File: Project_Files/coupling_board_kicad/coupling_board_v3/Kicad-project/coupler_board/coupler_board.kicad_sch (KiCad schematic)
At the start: 26 parts, among them IC1 ISO6741DWR, IC2 ISO6740FDWR, IC3 ISO6740FDWR, J1 Molex Microfit, J2 Conn_02x12_Odd_Even, J3 Molex6, J5 DB25_Socket, J7 Molex Microfit, J8 Molex Microfit, J9 Molex Microfit

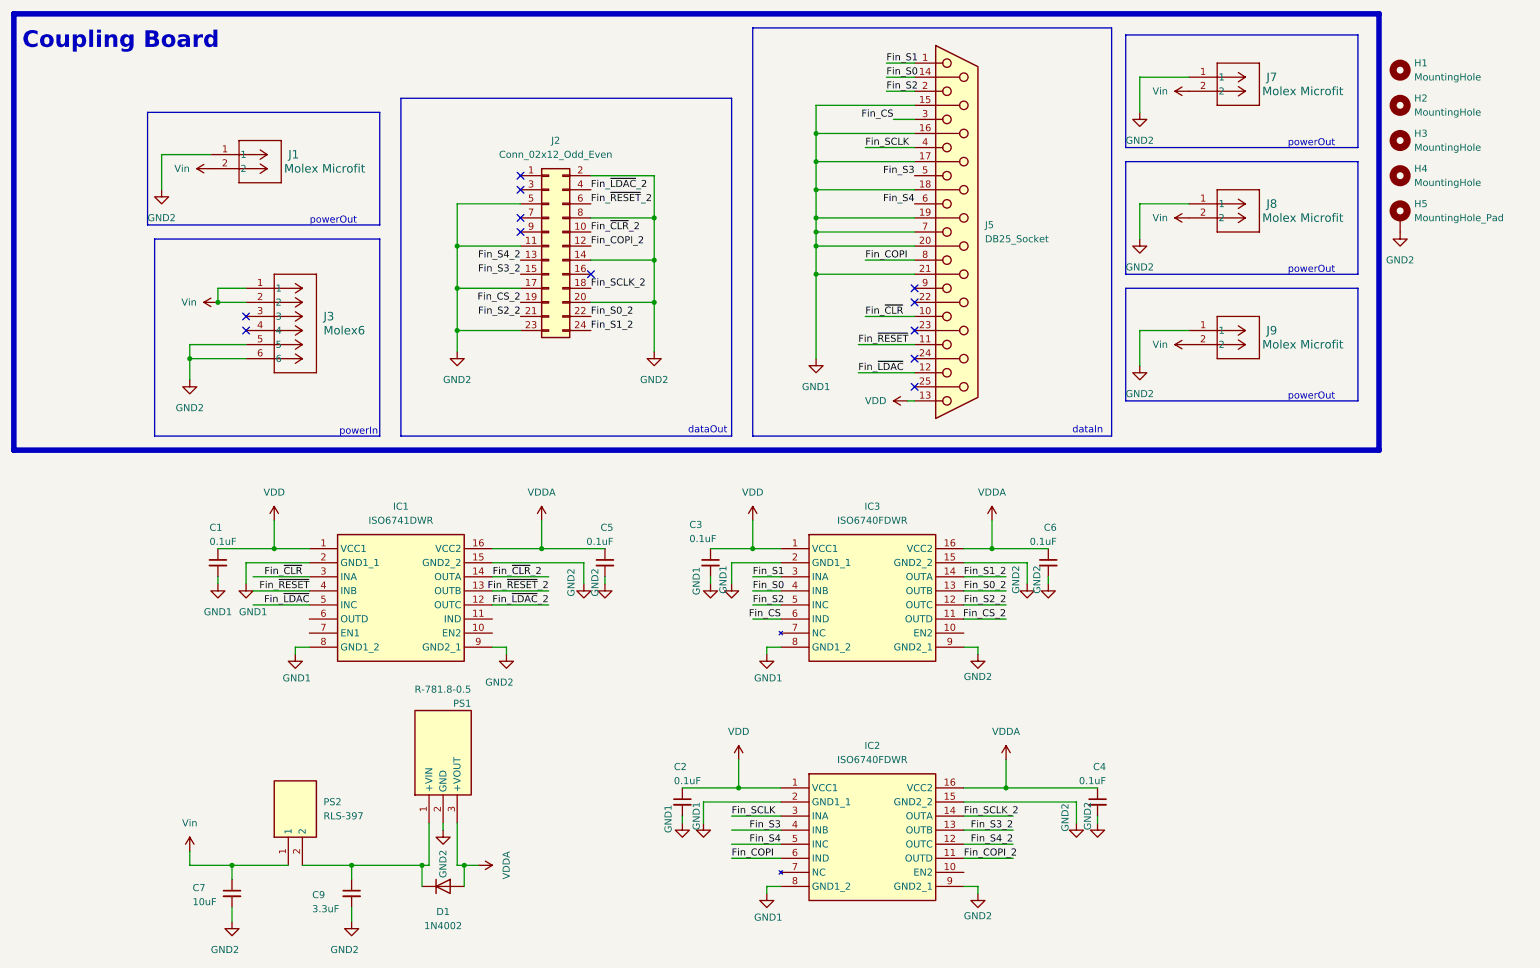
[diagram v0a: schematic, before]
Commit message: Updated design
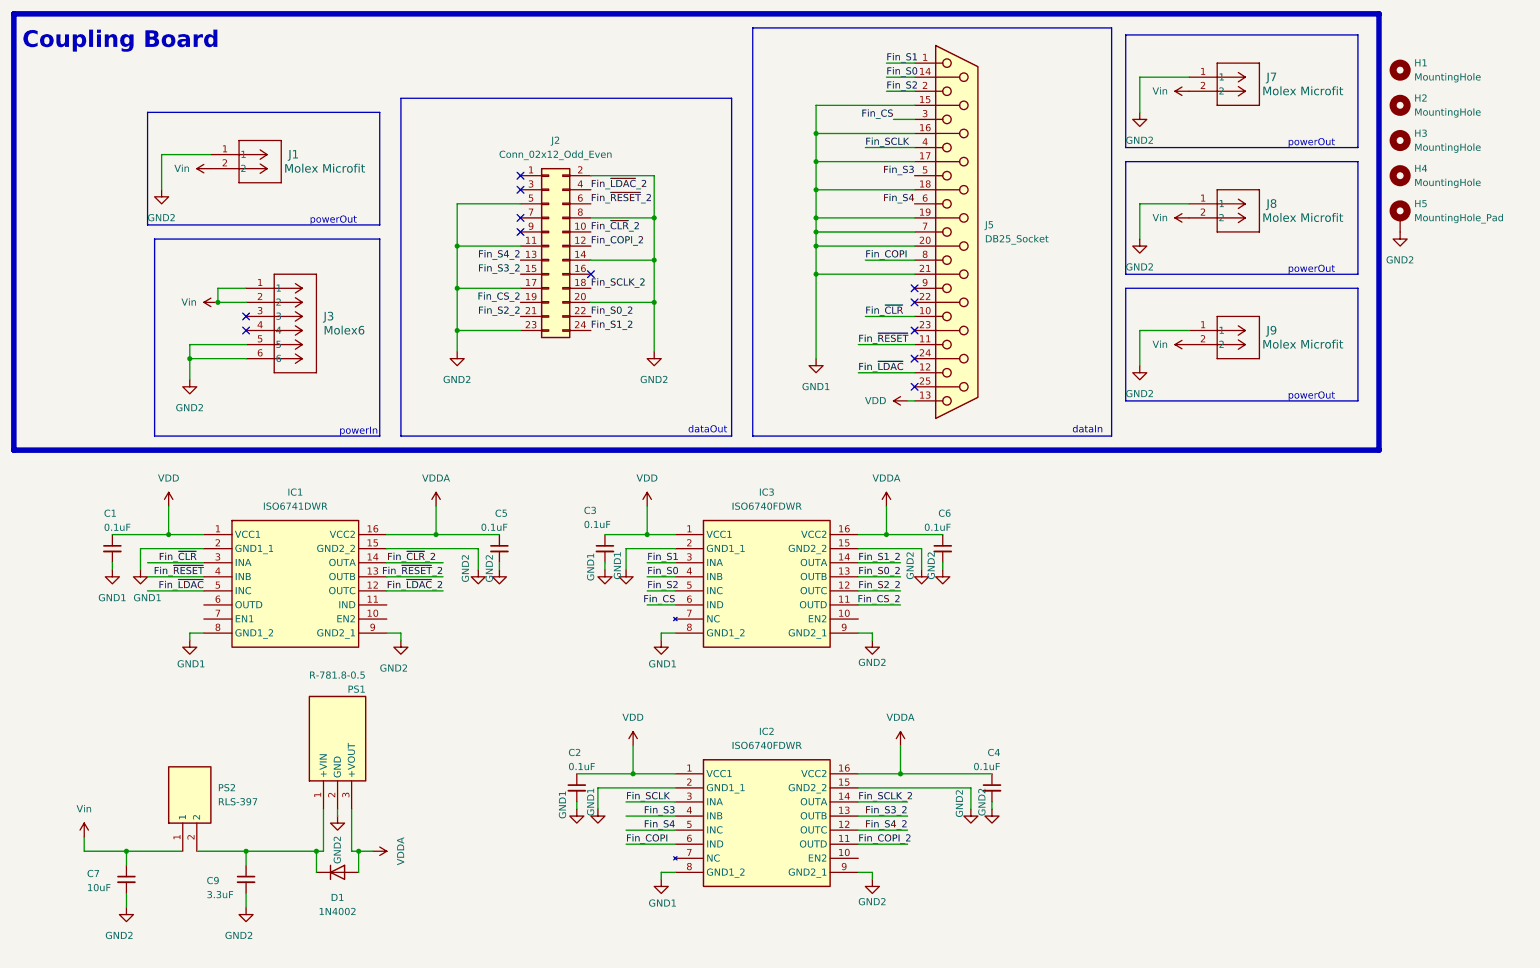
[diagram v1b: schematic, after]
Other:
- moved on the sheet: C1, C2, C3, C4, C5, C6, C7, C9, D1, IC1, IC2, IC3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
